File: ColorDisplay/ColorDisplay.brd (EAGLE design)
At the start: 36.3 x 29.8 mm, 16 parts, among them SW1 7914J-1-000E, SW2 7914J-1-000E, SW3 7914J-1-000E, U1 ER-OLED0.95-2C, U2 LM2665M6/NOPB, U3 ATSAMD21E18A-AU, U4 MIC5205-3.3YM5 TR

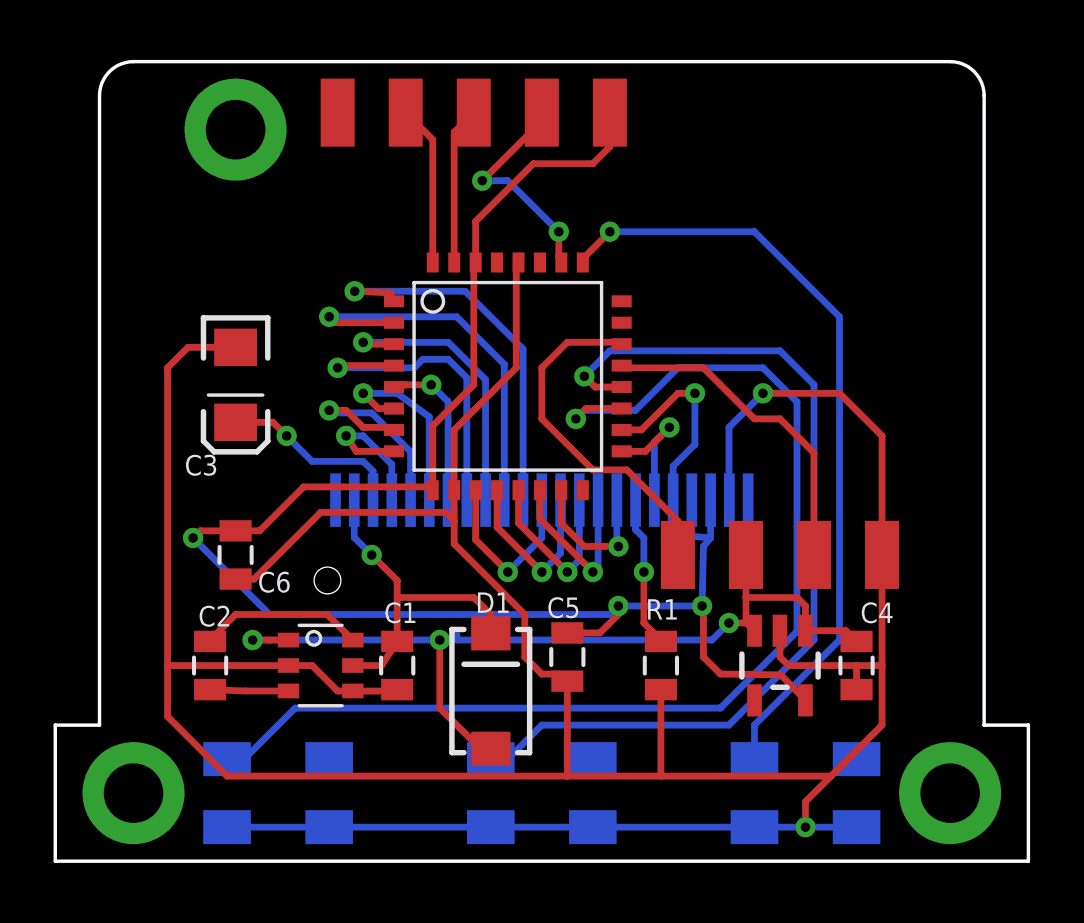
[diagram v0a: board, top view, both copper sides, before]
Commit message: Various updates
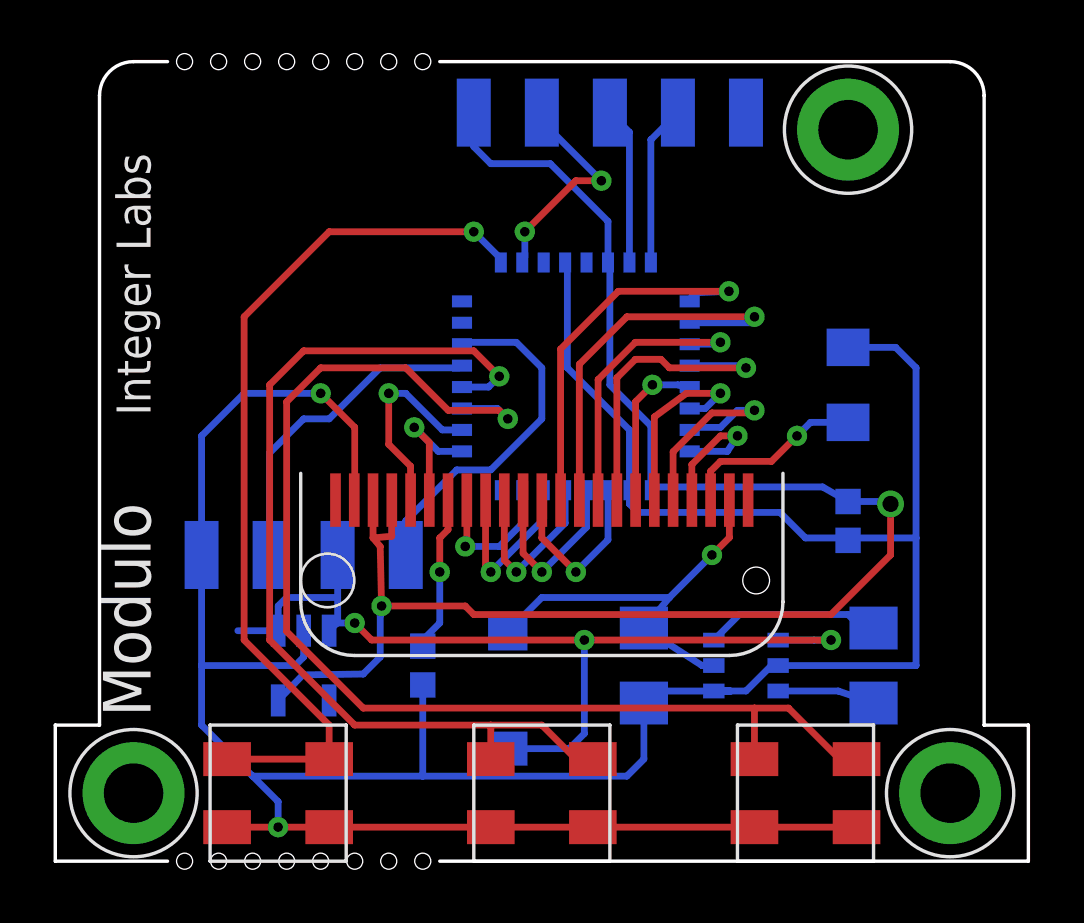
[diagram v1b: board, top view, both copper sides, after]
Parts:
- removed C5: 10uF, Modulo:0805
- removed C6: .47uF, Modulo:0805
- C1, C2: device Modulo:0805 -> Modulo:C1206
- C4: value 10uF -> 100nF; device Modulo:0805 -> Modulo:0603
- PCB1: value EXCLUDE -> DEVICE-PCB-TABS; device Modulo:DEVICE-PCB -> Modulo:DEVICE-PCB-TABS
- R1: device Modulo:0805 -> Modulo:0603
- U1: value ER-OLED0.95-2C -> LM2665M6/NOPB; device Modulo:FPC-24-REVERSE -> Modulo:SOT-26
- U2: value LM2665M6/NOPB -> ER-OLED0.95-2C; device Modulo:SOT-26 -> Modulo:FPC-24-REVERSE
- moved PCB1 35.6 mm to (0.00, 0.00), flipped to the top
- moved C2 24.8 mm to (30.2, 7.30), flipped to the bottom
- moved C3 22.9 mm to (29.2, 17.8), flipped to the bottom
- moved U4 17.8 mm to (8.89, 7.30), flipped to the bottom
- moved U2 10.9 mm to (17.8, 14.5), turned to 180 degrees
- moved U1 10.5 mm to (25.4, 7.30), turned to 270 degrees
- moved SW2 9.84 mm to (17.8, 2.54), flipped to the top
- moved SW3 9.84 mm to (27.6, 2.54), flipped to the top
- moved C1 9.21 mm to (21.6, 7.30), flipped to the bottom
- moved R1 8.89 mm to (13.3, 7.30), flipped to the bottom
- moved C4 5.41 mm to (29.2, 12.7), flipped to the bottom
- moved U3 2.54 mm to (19.1, 18.1), flipped to the bottom
- moved D1 0.64 mm to (16.5, 6.35), flipped to the bottom
- flipped SW1 to the top
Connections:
- net +10V: now also U1.5, U2.22; no longer U1.22, U2.5
- net +3.3V: now also C4.1, U2.3, U2.4; no longer C5.1, C6.1, U1.3, U1.4
- net +5V: now also U1.1; no longer C4.1, U2.1
- net BS0: now also U2.6; no longer U1.6
- net BS1: now also U2.5; no longer U1.5
- net BUTTON1: now also SW1.POS$1, SW1.POS$2; no longer SW2.POS$1, SW2.POS$2
- net BUTTON2: now also SW2.POS$1, SW2.POS$2; no longer SW3.POS$1, SW3.POS$2
- net BUTTON3: now also SW3.POS$1, SW3.POS$2; no longer SW1.POS$1, SW1.POS$2
- net CS: now also U2.8; no longer U1.8
- net D/C: now also U2.10; no longer U1.10
- net D0: now also U2.13; no longer U1.13
- net D1: now also U2.14; no longer U1.14
- net D2: now also U2.15; no longer U1.15
- net D3: now also U2.16; no longer U1.16
- net D4: now also U2.17; no longer U1.17
- net D5: now also U2.18; no longer U1.18
- net D6: now also U2.19; no longer U1.19
- net D7: now also U2.20; no longer U1.20
- net DISPLAY_RESET: now also U2.9; no longer U1.9
- net GND: now also U1.4; no longer C5.2, C6.2, U2.4
- net N$13: now also U1.6; no longer U2.6
- net N$14: now also U1.3; no longer U2.3
- net N$5: now also U2.21; no longer U1.21
- net N$8: now also U2.7; no longer U1.7
- net RD: now also U2.12; no longer U1.12
- net WR: now also U2.11; no longer U1.11
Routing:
- net GND: track 140.4 -> 121.9 mm
- net BUTTON1: track 29.3 -> 33.4 mm
- net +10V: track 12.5 -> 15.7 mm
- net BUTTON3: track 43.3 -> 45.2 mm
- net +3.3V: track 63.2 -> 61.8 mm, vias 3 -> 2
- net +5V: track 34.1 -> 35.4 mm
- net BUTTON2: track 34.5 -> 35.8 mm
- net N$13: track 6.17 -> 7.20 mm
- net N$14: track 2.93 -> 3.64 mm
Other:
- outline, holes or cut-outs redrawn
